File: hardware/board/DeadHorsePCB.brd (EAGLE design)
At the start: 67.8 x 63.2 mm, 23 parts, among them J1 DIN5, Q1 BSS138, Q2 BSS138

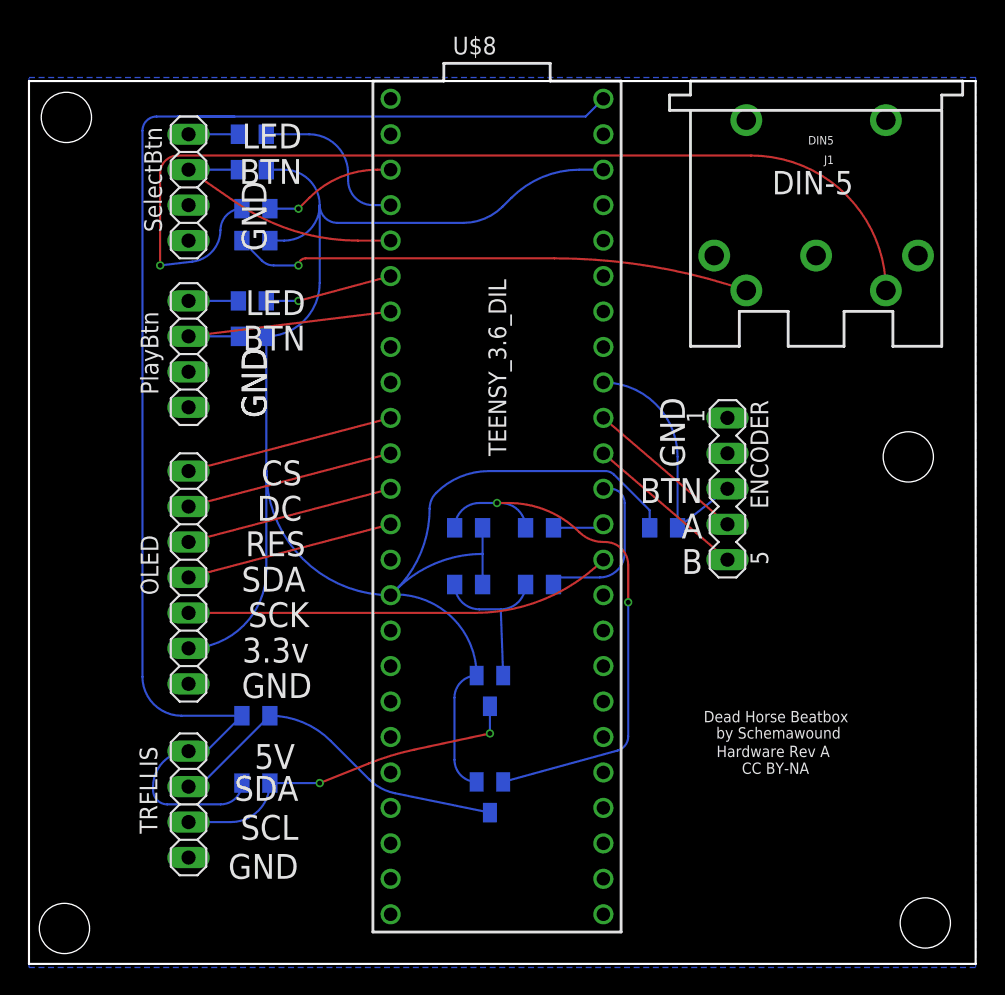
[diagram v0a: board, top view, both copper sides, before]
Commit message: Ripup
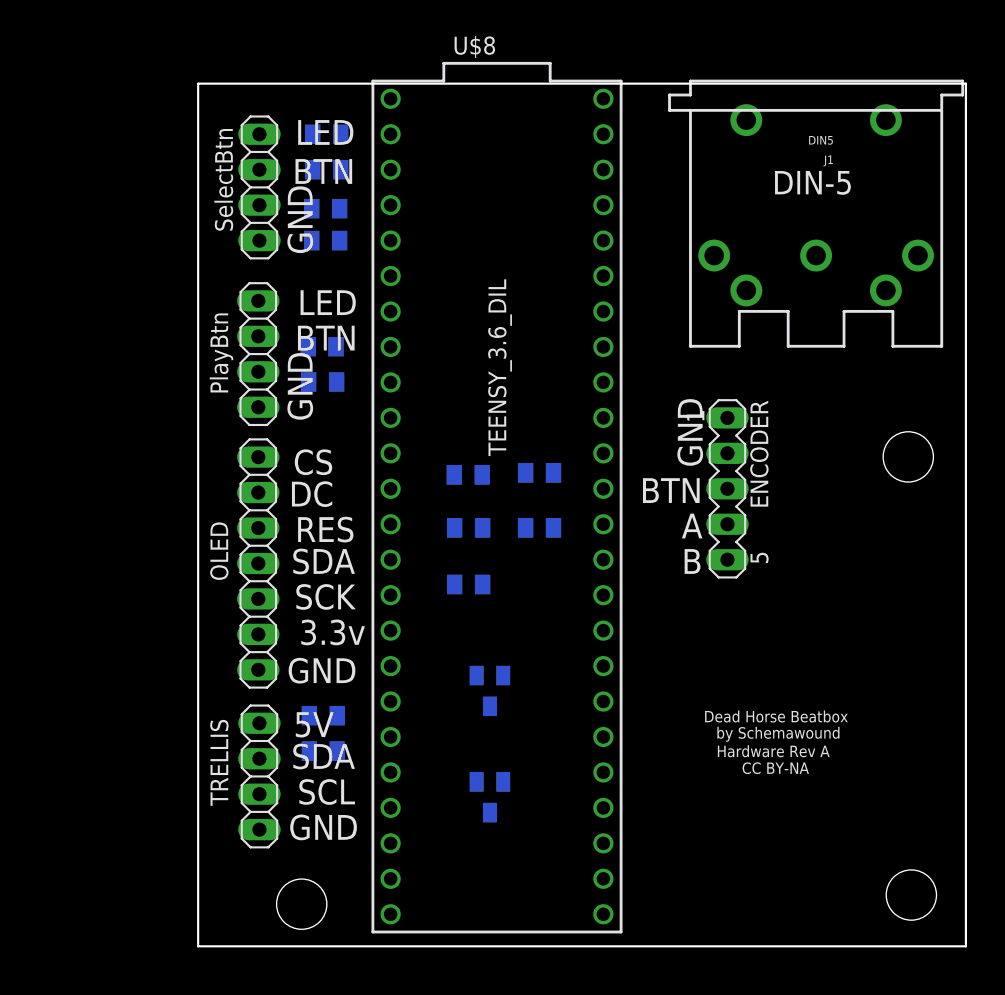
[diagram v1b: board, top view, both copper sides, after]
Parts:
- moved R12 14.5 mm to (61.9, 50.3), turned to 180 degrees
- moved R6 8.00 mm to (67.1, 50.4)
- moved R9 6.00 mm to (51.5, 56.9)
- moved R8 5.98 mm to (51.5, 59.5)
- moved TRELLIS 5.46 mm to (47.0, 28.7)
- moved R3 5.34 mm to (51.6, 30.5)
- moved R10 5.33 mm to (51.8, 74.7)
- moved R11 5.33 mm to (51.8, 72.1)
- moved OLED 5.10 mm to (46.9, 43.9)
- moved SELECT_BUTTON 5.08 mm to (47.0, 70.9)
- moved PLAY_BUTTON 5.00 mm to (46.9, 58.9)
- moved R13 5.00 mm to (51.7, 67.1)
- moved R7 5.00 mm to (51.7, 69.3)
- moved R2 4.83 mm to (51.6, 33.0)
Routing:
- net 3.3V: track 133.7 -> 0.00 mm
- net VIN: track 101.6 -> 0.00 mm
- net N$4: track 70.6 -> 0.00 mm, vias 1 -> 0
- net N$5: track 39.2 -> 0.00 mm, vias 2 -> 0
- net N$3: track 37.2 -> 0.00 mm, vias 1 -> 0
- net SCK: track 30.5 -> 0.00 mm
- net N$2: track 25.6 -> 0.00 mm
- net N$8: track 25.2 -> 0.00 mm, vias 2 -> 0
- net N$22: track 19.2 -> 0.00 mm
- net N$14: track 18.2 -> 0.00 mm
- net N$20: track 17.2 -> 0.00 mm
- net SDA: track 15.0 -> 0.00 mm
- net RES: track 15.0 -> 0.00 mm
- net DC: track 15.0 -> 0.00 mm
- net CS: track 15.0 -> 0.00 mm
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- removed copper zone on layer 16, net GND
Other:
- board size 67.8 x 63.2 mm -> 55 x 61.8 mm
